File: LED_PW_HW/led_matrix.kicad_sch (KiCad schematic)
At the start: 79 parts, among them U1 IS31FL3746A

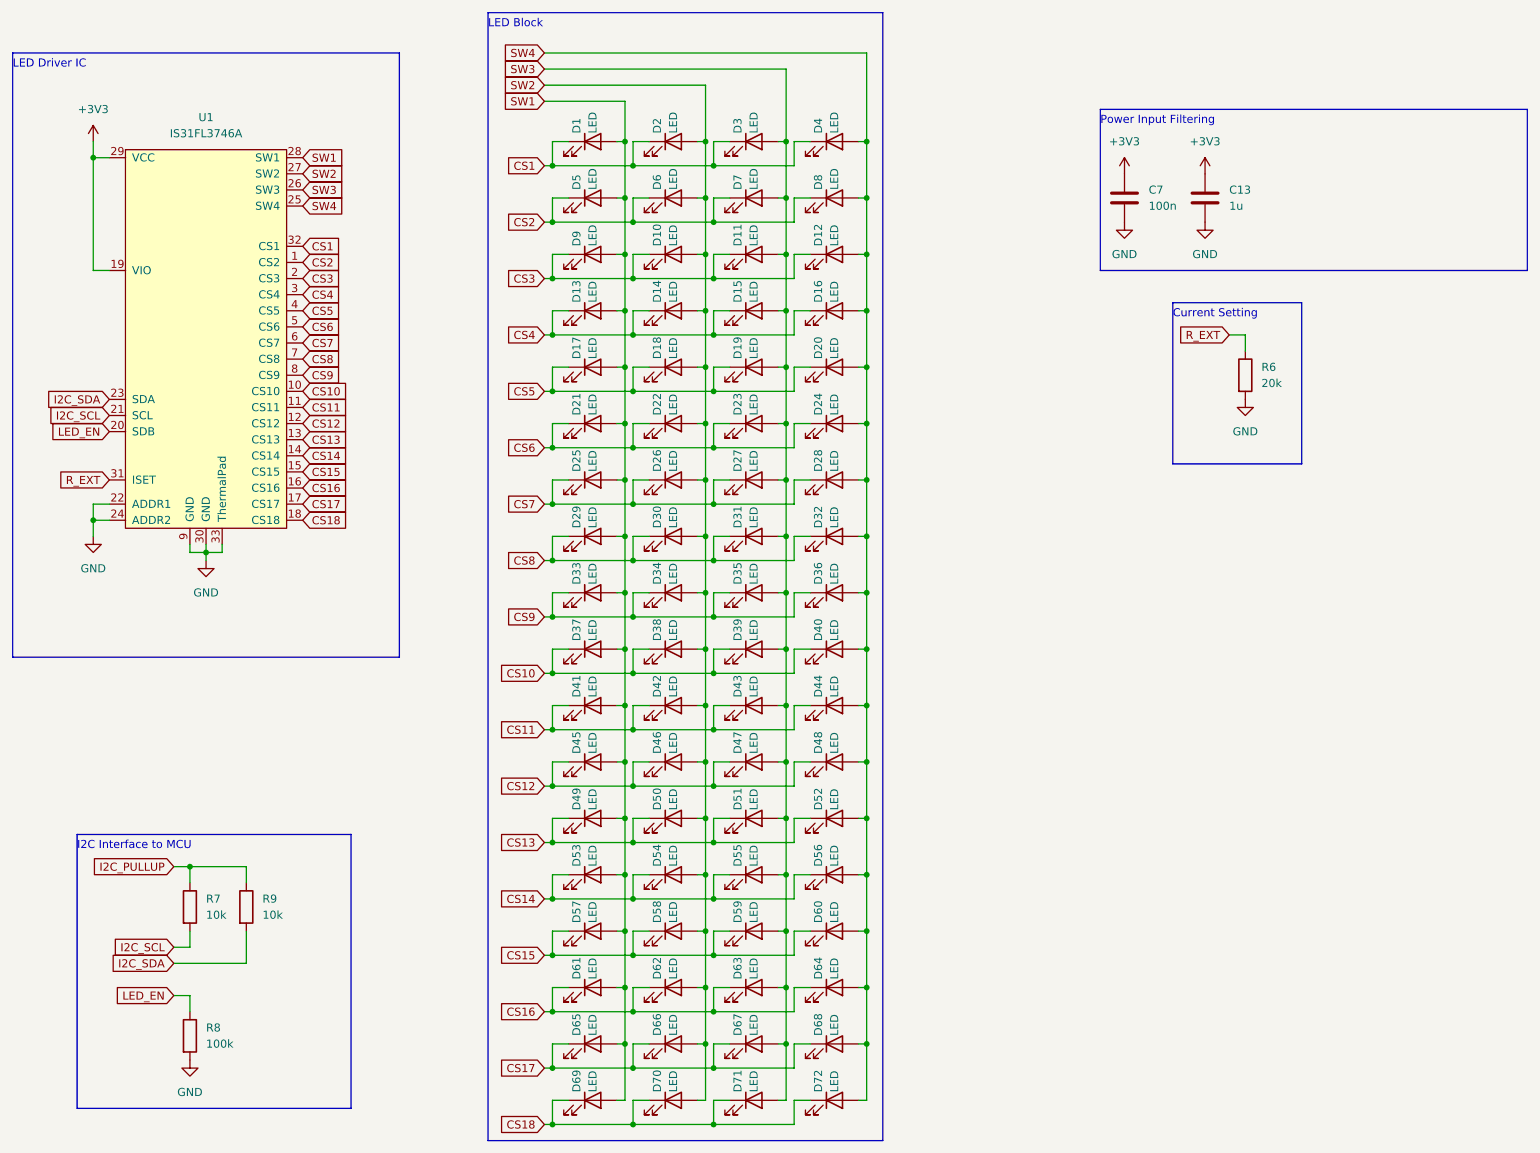
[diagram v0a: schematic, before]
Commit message: new version
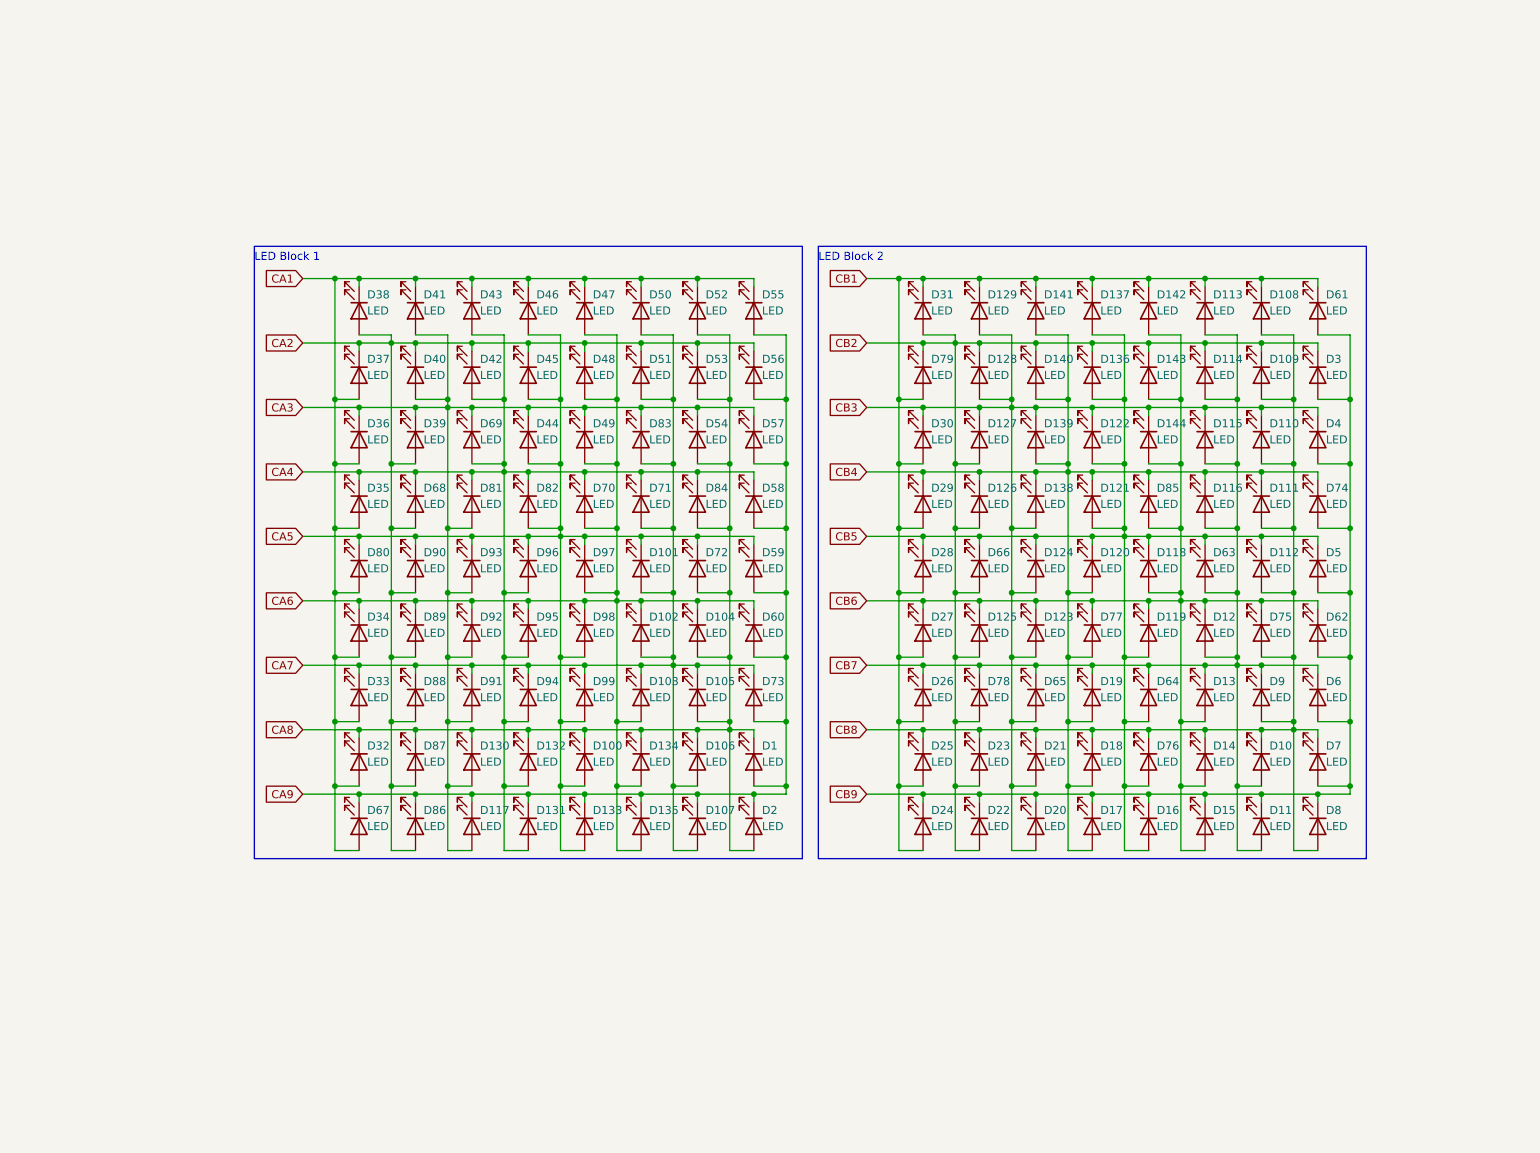
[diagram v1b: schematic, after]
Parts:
- removed C13: 1u, Capacitor_SMD:C_0603_1608Metric_Pad1.08x0.95mm_HandSolder, symbol Device:C
- removed C7: 100n, Capacitor_SMD:C_0603_1608Metric_Pad1.08x0.95mm_HandSolder, symbol Device:C
- removed R6: 20k, Resistor_SMD:R_0603_1608Metric_Pad0.98x0.95mm_HandSolder, symbol Device:R
- removed R7, R9: 10k, Resistor_SMD:R_0603_1608Metric_Pad0.98x0.95mm_HandSolder, symbol Device:R
- removed R8: 100k, Resistor_SMD:R_0603_1608Metric_Pad0.98x0.95mm_HandSolder, symbol Device:R
- removed U1: IS31FL3746A, LED_Clock_HW:QFN-32_EP_4x4_Pitch0.4mm, symbol LED_Clock_HW:IS31FL3746A
- added D100, D101, D102, D103, D104, D105, D106, D107, D108, D109, D110, D111, D112, D113, D114, D115, D116, D117, D118, D119, D120, D121, D122, D123, D124, D125, D126, D127, D128, D129, D130, D131, D132, D133, D134, D135, D136, D137, D138, D139, D140, D141, D142, D143, D144, D73, D74, D75, D76, D77, D78, D79, D80, D81, D82, D83, D84, D85, D86, D87, D88, D89, D90, D91, D92, D93, D94, D95, D96, D97, D98, D99: LED, LED_SMD:LED_0603_1608Metric_Pad1.05x0.95mm_HandSolder, symbol Device:LED
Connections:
- removed net CS1: D1.1 (K), D2.1 (K), D3.1 (K), D4.1 (K)
- net CS10 renamed CA2
- net CA2: now also D38.2 (A), D39.2 (A), D42.1 (K), D45.1 (K), D48.1 (K), D51.1 (K), D53.1 (K), D56.1 (K), D68.2 (A), D86.2 (A), D87.2 (A), D88.2 (A), D89.2 (A), D90.2 (A); no longer D38.1 (K), D39.1 (K)
- net CS11 renamed CA1
- net CA1: now also D32.2 (A), D33.2 (A), D34.2 (A), D35.2 (A), D36.2 (A), D37.2 (A), D38.1 (K), D46.1 (K), D47.1 (K), D50.1 (K), D52.1 (K), D55.1 (K), D67.2 (A), D80.2 (A); no longer D42.1 (K), D44.1 (K)
- removed net CS12: D45.1 (K), D46.1 (K), D47.1 (K), D48.1 (K)
- removed net CS13: D49.1 (K), D50.1 (K), D51.1 (K), D52.1 (K)
- removed net CS14: D53.1 (K), D54.1 (K), D55.1 (K), D56.1 (K)
- removed net CS15: D57.1 (K), D58.1 (K), D59.1 (K), D60.1 (K)
- removed net CS16: D61.1 (K), D62.1 (K), D63.1 (K), D64.1 (K)
- removed net CS17: D65.1 (K), D66.1 (K), D67.1 (K), D68.1 (K)
- net CS18 renamed CA4
- net CA4: now also D35.1 (K), D42.2 (A), D43.2 (A), D58.1 (K), D68.1 (K), D69.2 (A), D131.2 (A), D132.2 (A), D81.1 (K), D82.1 (K), D84.1 (K), D94.2 (A), D95.2 (A), D96.2 (A); no longer D69.1 (K), D72.1 (K)
- removed net CS2: D5.1 (K), D6.1 (K), D7.1 (K), D8.1 (K)
- removed net CS3: D10.1 (K), D11.1 (K), D12.1 (K), D9.1 (K)
- net CS4 renamed CB9
- net CB9: now also D11.1 (K), D17.1 (K), D20.1 (K), D22.1 (K), D24.1 (K), D3.2 (A), D4.2 (A), D5.2 (A), D6.2 (A), D61.2 (A), D62.2 (A), D7.2 (A), D8.1 (K), D74.2 (A); no longer D13.1 (K), D14.1 (K)
- removed net CS5: D17.1 (K), D18.1 (K), D19.1 (K), D20.1 (K)
- net CS6 renamed CB8
- net CB8: now also D10.1 (K), D14.1 (K), D18.1 (K), D25.1 (K), D7.1 (K), D8.2 (A), D9.2 (A), D108.2 (A), D109.2 (A), D110.2 (A), D111.2 (A), D112.2 (A), D75.2 (A), D76.1 (K); no longer D22.1 (K), D24.1 (K)
- removed net CS7: D25.1 (K), D26.1 (K), D27.1 (K), D28.1 (K)
- removed net CS8: D29.1 (K), D30.1 (K), D31.1 (K), D32.1 (K)
- removed net CS9: D33.1 (K), D34.1 (K), D35.1 (K), D36.1 (K)
- removed net SW1: D1.2 (A), D13.2 (A), D17.2 (A), D21.2 (A), D25.2 (A), D29.2 (A), D33.2 (A), D37.2 (A), D41.2 (A), D45.2 (A), D49.2 (A), D5.2 (A), D53.2 (A), D57.2 (A), D61.2 (A), D65.2 (A), D69.2 (A), D9.2 (A)
- removed net SW2: D10.2 (A), D14.2 (A), D18.2 (A), D2.2 (A), D22.2 (A), D26.2 (A), D30.2 (A), D34.2 (A), D38.2 (A), D42.2 (A), D46.2 (A), D50.2 (A), D54.2 (A), D58.2 (A), D6.2 (A), D62.2 (A), D66.2 (A), D70.2 (A)
- removed net SW3: D11.2 (A), D15.2 (A), D19.2 (A), D23.2 (A), D27.2 (A), D3.2 (A), D31.2 (A), D35.2 (A), D39.2 (A), D43.2 (A), D47.2 (A), D51.2 (A), D55.2 (A), D59.2 (A), D63.2 (A), D67.2 (A), D7.2 (A), D71.2 (A)
- removed net SW4: D12.2 (A), D16.2 (A), D20.2 (A), D24.2 (A), D28.2 (A), D32.2 (A), D36.2 (A), D4.2 (A), D40.2 (A), D44.2 (A), D48.2 (A), D52.2 (A), D56.2 (A), D60.2 (A), D64.2 (A), D68.2 (A), D72.2 (A), D8.2 (A)
- new net CA3: D117.2 (A), D130.2 (A), D36.1 (K), D39.1 (K), D40.2 (A), D41.2 (A), D44.1 (K), D49.1 (K), D54.1 (K), D57.1 (K), D69.1 (K), D81.2 (A), D83.1 (K), D91.2 (A), D92.2 (A), D93.2 (A)
- new net CA5: D100.2 (A), D101.1 (K), D133.2 (A), D44.2 (A), D45.2 (A), D46.2 (A), D59.1 (K), D72.1 (K), D80.1 (K), D82.2 (A), D90.1 (K), D93.1 (K), D96.1 (K), D97.1 (K), D98.2 (A), D99.2 (A)
- new net CA6: D102.1 (K), D103.2 (A), D104.1 (K), D134.2 (A), D135.2 (A), D34.1 (K), D47.2 (A), D48.2 (A), D49.2 (A), D60.1 (K), D70.2 (A), D89.1 (K), D92.1 (K), D95.1 (K), D97.2 (A), D98.1 (K)
- new net CA7: D101.2 (A), D102.2 (A), D103.1 (K), D105.1 (K), D106.2 (A), D107.2 (A), D33.1 (K), D50.2 (A), D51.2 (A), D71.2 (A), D73.1 (K), D83.2 (A), D88.1 (K), D91.1 (K), D94.1 (K), D99.1 (K)
- new net CA8: D1.1 (K), D100.1 (K), D104.2 (A), D105.2 (A), D106.1 (K), D130.1 (K), D132.1 (K), D134.1 (K), D2.2 (A), D32.1 (K), D52.2 (A), D53.2 (A), D54.2 (A), D72.2 (A), D84.2 (A), D87.1 (K)
- new net CA9: D1.2 (A), D107.1 (K), D117.1 (K), D131.1 (K), D133.1 (K), D135.1 (K), D2.1 (K), D55.2 (A), D56.2 (A), D57.2 (A), D58.2 (A), D59.2 (A), D60.2 (A), D67.1 (K), D73.2 (A), D86.1 (K)
- new net CB1: D108.1 (K), D113.1 (K), D129.1 (K), D137.1 (K), D141.1 (K), D142.1 (K), D24.2 (A), D25.2 (A), D26.2 (A), D27.2 (A), D28.2 (A), D29.2 (A), D30.2 (A), D31.1 (K), D61.1 (K), D79.2 (A)
- new net CB2: D109.1 (K), D114.1 (K), D125.2 (A), D126.2 (A), D127.2 (A), D128.1 (K), D136.1 (K), D140.1 (K), D143.1 (K), D22.2 (A), D23.2 (A), D3.1 (K), D31.2 (A), D66.2 (A), D78.2 (A), D79.1 (K)
- new net CB3: D110.1 (K), D115.1 (K), D122.1 (K), D123.2 (A), D124.2 (A), D127.1 (K), D128.2 (A), D129.2 (A), D138.2 (A), D139.1 (K), D144.1 (K), D20.2 (A), D21.2 (A), D30.1 (K), D4.1 (K), D65.2 (A)
- new net CB4: D111.1 (K), D116.1 (K), D120.2 (A), D121.1 (K), D126.1 (K), D138.1 (K), D139.2 (A), D140.2 (A), D141.2 (A), D17.2 (A), D18.2 (A), D19.2 (A), D29.1 (K), D74.1 (K), D77.2 (A), D85.1 (K)
- new net CB5: D112.1 (K), D118.1 (K), D119.2 (A), D120.1 (K), D121.2 (A), D122.2 (A), D124.1 (K), D136.2 (A), D137.2 (A), D16.2 (A), D28.1 (K), D5.1 (K), D63.1 (K), D64.2 (A), D66.1 (K), D76.2 (A)
- new net CB6: D118.2 (A), D119.1 (K), D12.1 (K), D123.1 (K), D125.1 (K), D13.2 (A), D14.2 (A), D142.2 (A), D143.2 (A), D144.2 (A), D15.2 (A), D27.1 (K), D62.1 (K), D75.1 (K), D77.1 (K), D85.2 (A)
- new net CB7: D10.2 (A), D11.2 (A), D113.2 (A), D114.2 (A), D115.2 (A), D116.2 (A), D12.2 (A), D13.1 (K), D19.1 (K), D26.1 (K), D6.1 (K), D63.2 (A), D64.1 (K), D65.1 (K), D78.1 (K), D9.1 (K)
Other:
- note added: "LED Block 1"
- note added: "LED Block 2"
- note removed: "Current Setting"
- note removed: "I2C Interface to MCU"
- note removed: "LED Block"
- note removed: "LED Driver IC"
- note removed: "Power Input Filtering"
- moved on the sheet: D1
